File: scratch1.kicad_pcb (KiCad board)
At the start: 2 copper layers, 24 parts, among them J1 USB_B_Micro, SW1 SW_Push, U1 ATmega32U4-A, Y1 16MHz

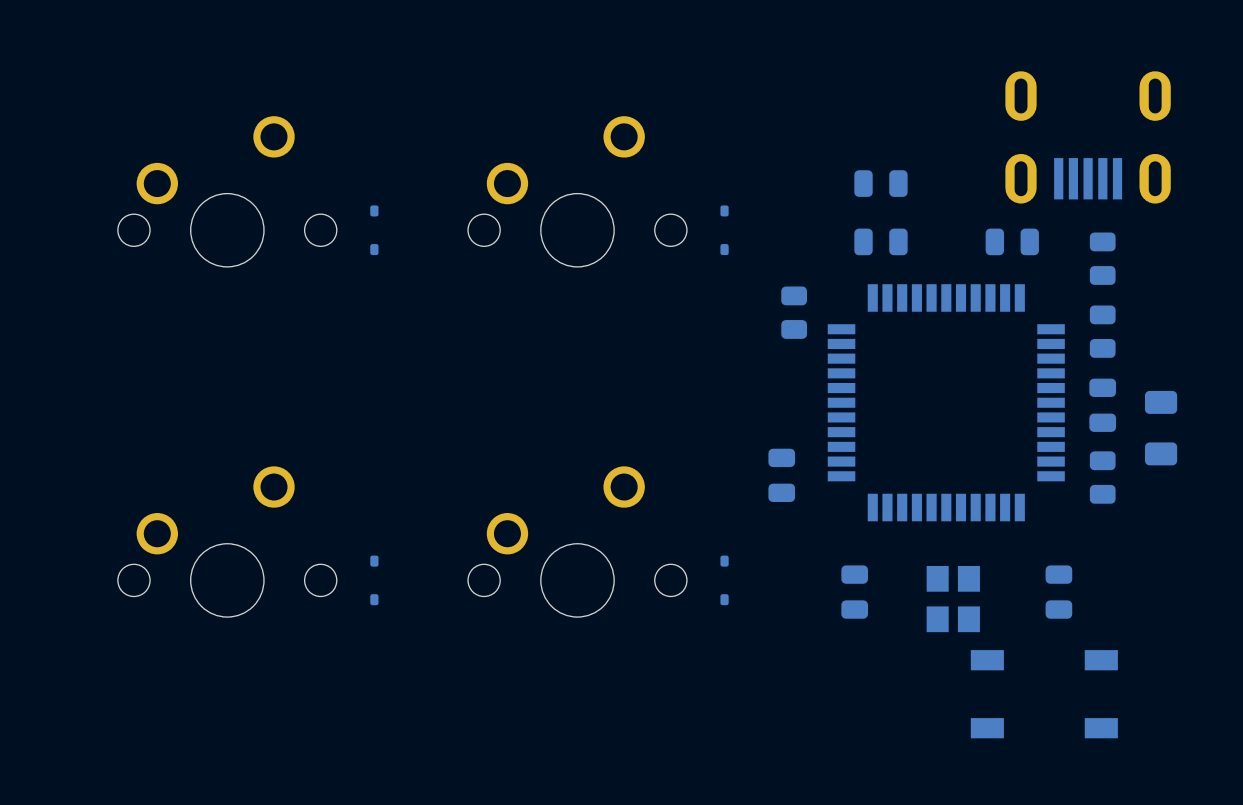
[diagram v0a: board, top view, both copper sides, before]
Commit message: finished routing
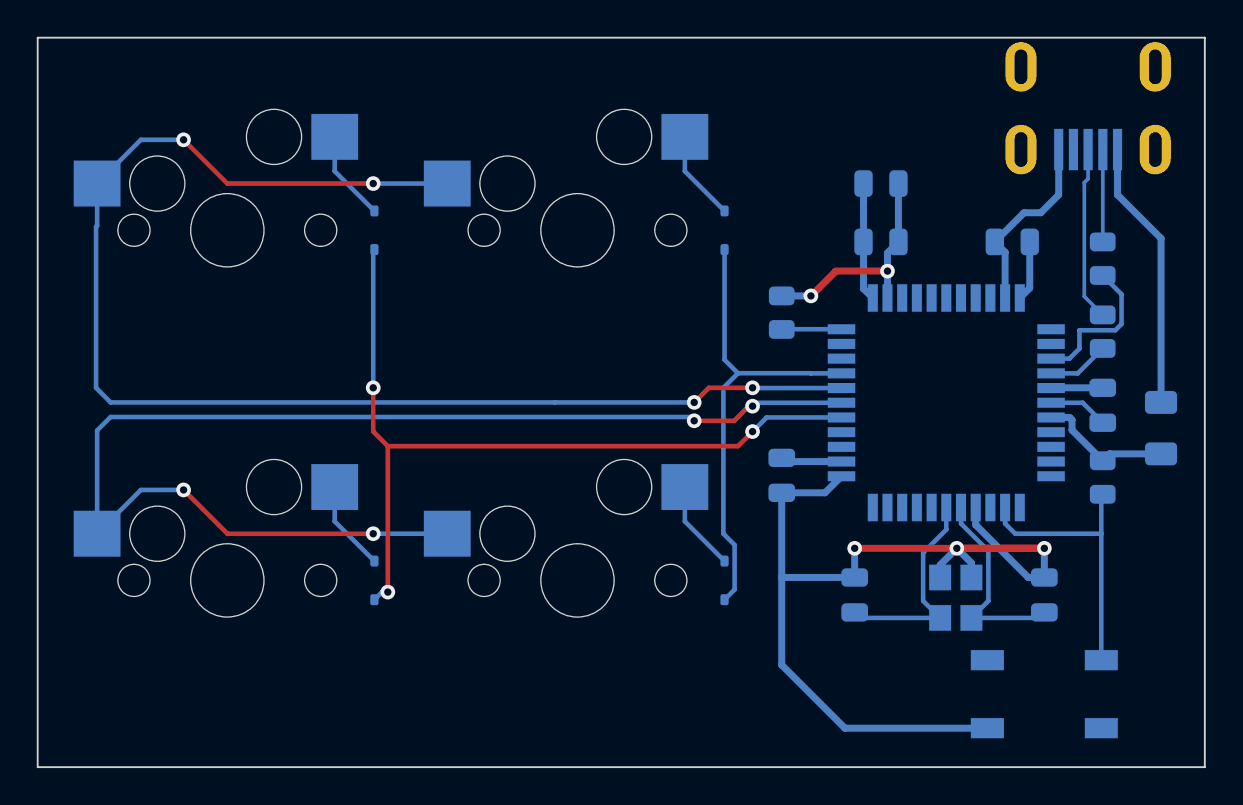
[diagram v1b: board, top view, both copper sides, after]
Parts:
- MX1, MX2, MX3, MX4: footprint MX_Only:MXOnly-1U-NoLED -> MX_Only:MXOnly-1U-Hotswap
- moved C4 11.1 mm to (81.8, 76.4), turned to -90 degrees
- moved C5 10.3 mm to (92.1, 76.4), turned to -90 degrees
- moved J1 1.59 mm to (94.5, 47.6)
- moved R4 0.68 mm to (77.8, 61.0)
- moved Y1 0.15 mm to (87.3, 76.5), turned to 90 degrees
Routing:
- net GND: track 0.00 -> 83.5 mm, vias 0 -> 5
- net COL0: track 0.00 -> 73.4 mm, vias 0 -> 4
- net COL1: track 0.00 -> 68.3 mm, vias 0 -> 4
- net ROW0: track 0.00 -> 45.2 mm, vias 0 -> 3
- net ROW1: track 0.00 -> 25.8 mm
- net +5V: track 0.00 -> 20.5 mm
- net Net-(U1-~{RESET}): track 0.00 -> 15.4 mm
- net VCC: track 0.00 -> 14.7 mm
- net Net-(U1-XTAL1): track 0.00 -> 11.7 mm
- net Net-(U1-XTAL2): track 0.00 -> 11.1 mm
- net D+: track 0.00 -> 9.49 mm
- net Net-(U1-D-): track 0.00 -> 8.27 mm
- net D-: track 0.00 -> 5.03 mm
- net Net-(D4-A): track 0.00 -> 4.92 mm
- net Net-(D2-A): track 0.00 -> 4.92 mm
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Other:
- board outline added: 63.5 x 39.7 mm
